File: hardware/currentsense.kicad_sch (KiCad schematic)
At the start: 12 parts, among them U801 CC6900SO-5A, U802 CC6900SO-5A, U803 CC6900SO-5A

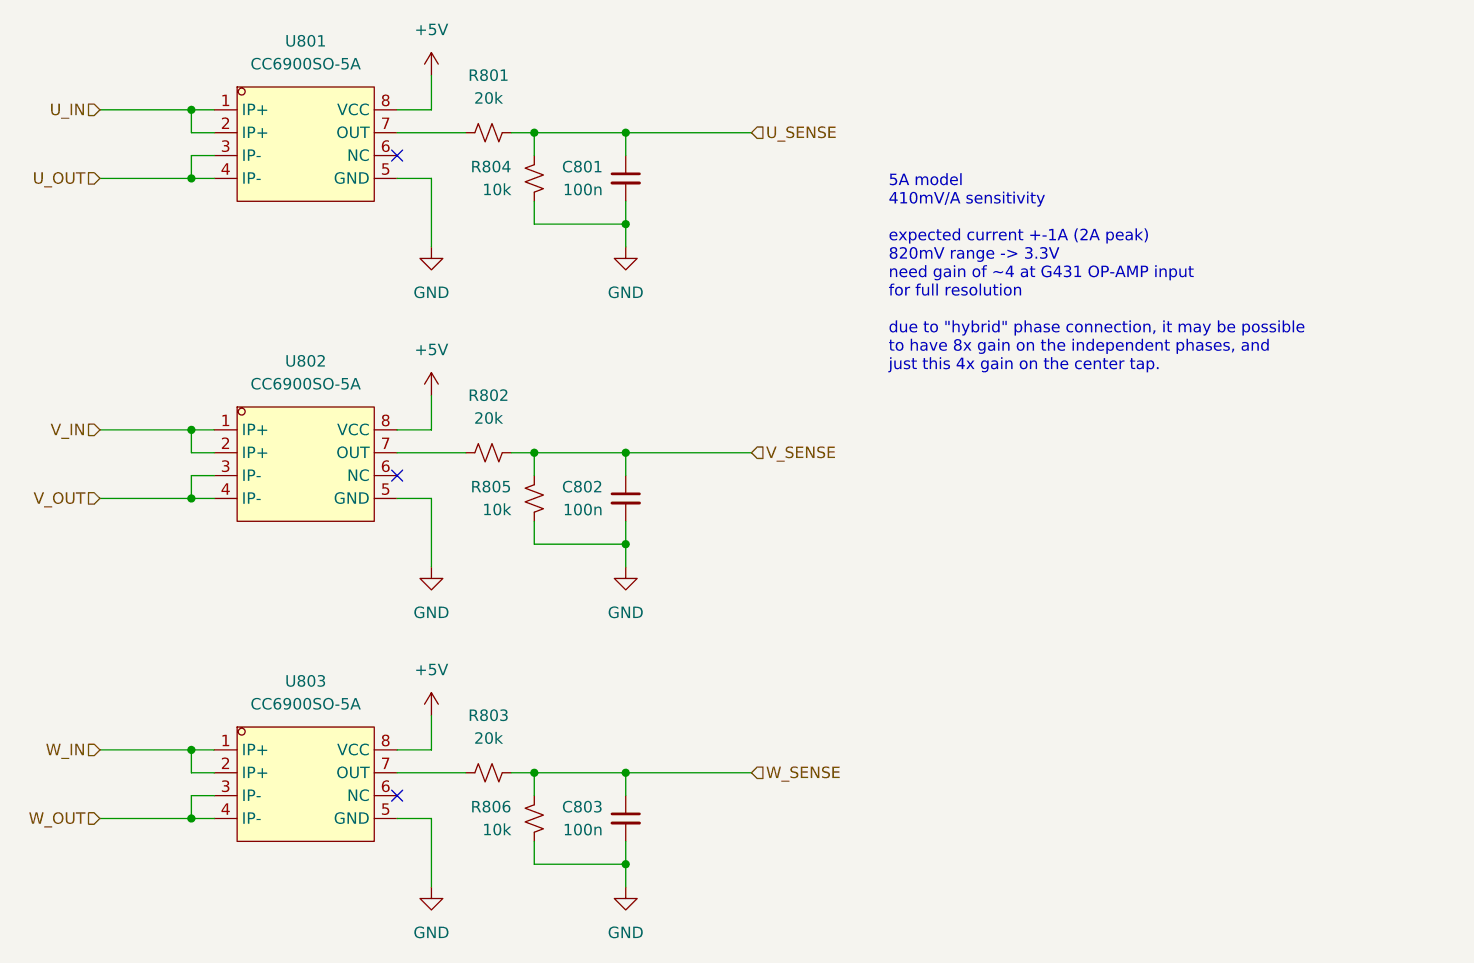
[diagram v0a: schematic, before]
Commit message: try new driver
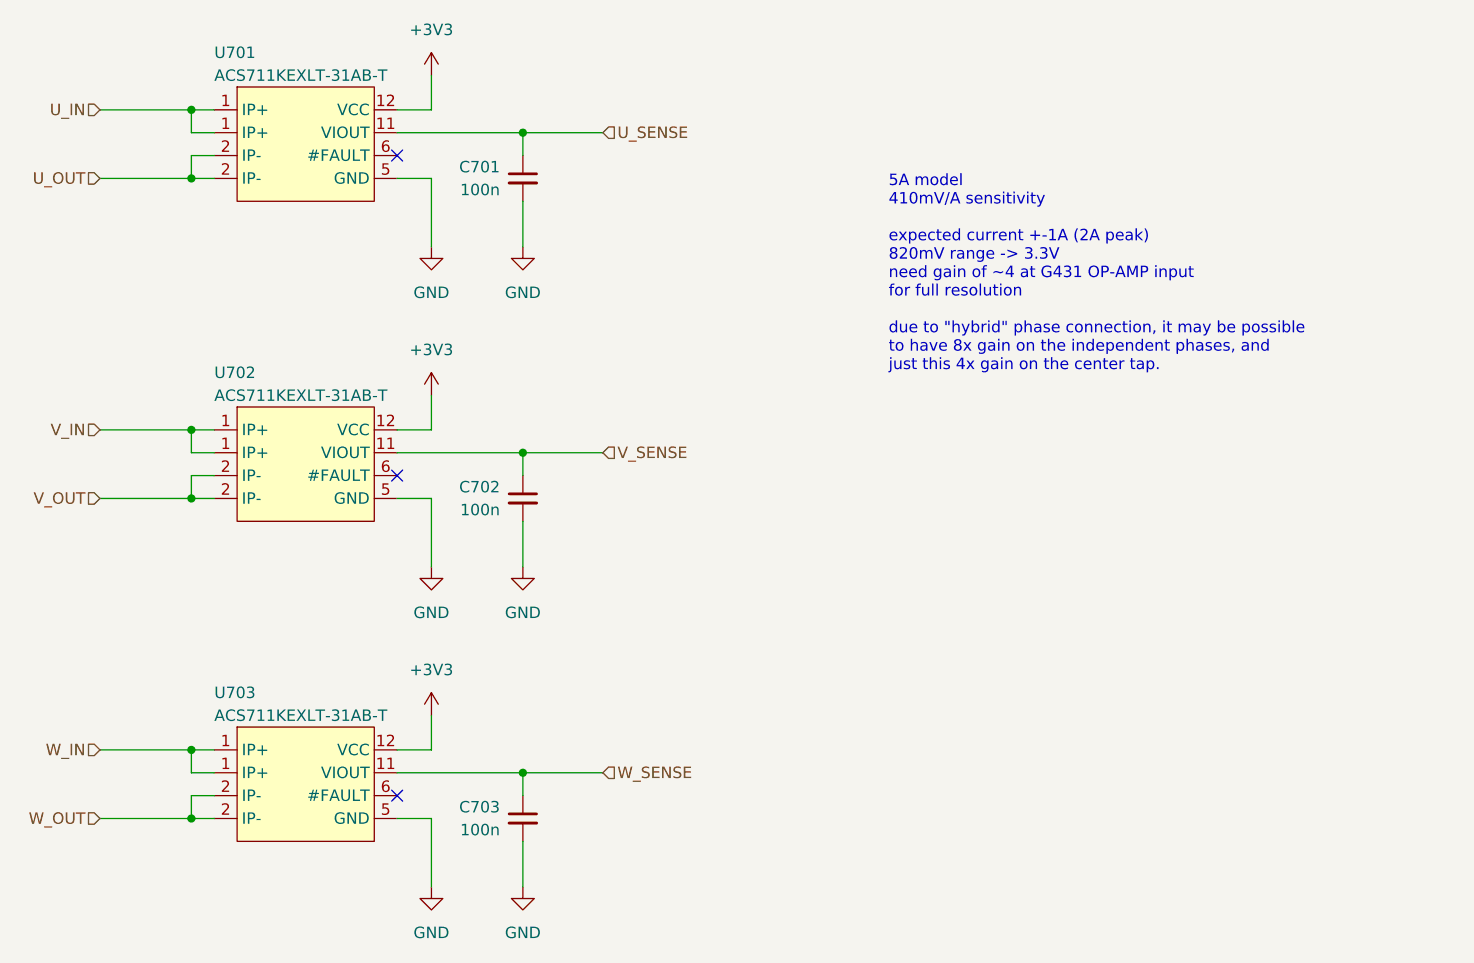
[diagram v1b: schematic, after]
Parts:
- removed R801, R802, R803: 20k, Resistor_SMD:R_0402_1005Metric, symbol Device:R_Small_US
- removed R804, R805, R806: 10k, Resistor_SMD:R_0402_1005Metric, symbol Device:R_Small_US
- removed U801, U802, U803: CC6900SO-5A, easyeda2kicad:SOP-8_L4.9-W3.9-P1.27-LS6.0-BL, symbol easyeda2kicad:CC6900SO-5A
- added U701, U702, U703: ACS711KEXLT-31AB-T, easyeda2kicad:IC-SMD_ACS711KEXLT-15AB-T, symbol easyeda2kicad:ACS711KEXLT-31AB-T
- renumbered C801 to C701, C802 to C702, C803 to C703
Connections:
- net GND: now also U701.10 (NC), U701.5 (GND), U701.7 (NC), U701.8 (NC), U701.9 (NC), U702.10 (NC), U702.5 (GND), U702.7 (NC), U702.8 (NC), U702.9 (NC), U703.10 (NC), U703.5 (GND), U703.7 (NC), U703.8 (NC), U703.9 (NC)
- net U_IN: now also U701.1 (IP+)
- net U_OUT: now also U701.2 (IP-)
- net U_SENSE: now also U701.11 (VIOUT)
- net V_IN: now also U702.1 (IP+)
- net V_OUT: now also U702.2 (IP-)
- net V_SENSE: now also U702.11 (VIOUT)
- net W_IN: now also U703.1 (IP+)
- net W_OUT: now also U703.2 (IP-)
- net W_SENSE: now also U703.11 (VIOUT)
- new net +3V3: U701.12 (VCC), U702.12 (VCC), U703.12 (VCC)
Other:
- moved on the sheet: C701, C702, C703
